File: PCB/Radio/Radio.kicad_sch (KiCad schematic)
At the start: 35 parts, among them J1 hc 12, J2 USB_C_Receptacle_USB2.0_16P, J3 seting, J4 config, J5 seting, J6 seting, J7 Conn_01x07_Pin, SW1 RotaryEncoder_Switch_MP, SW2 talk2push, SW3 SW_Push_45deg, SW4 SW_Push_45deg, SW5 SW_Push_45deg, SW6 SW_Push_45deg, SW7 RESET, SW8 RESET, U1 NRF24L01_Breakout, U2 ESP32-WROOM-32, U3 AMS1117-3.3, U4 CH340C

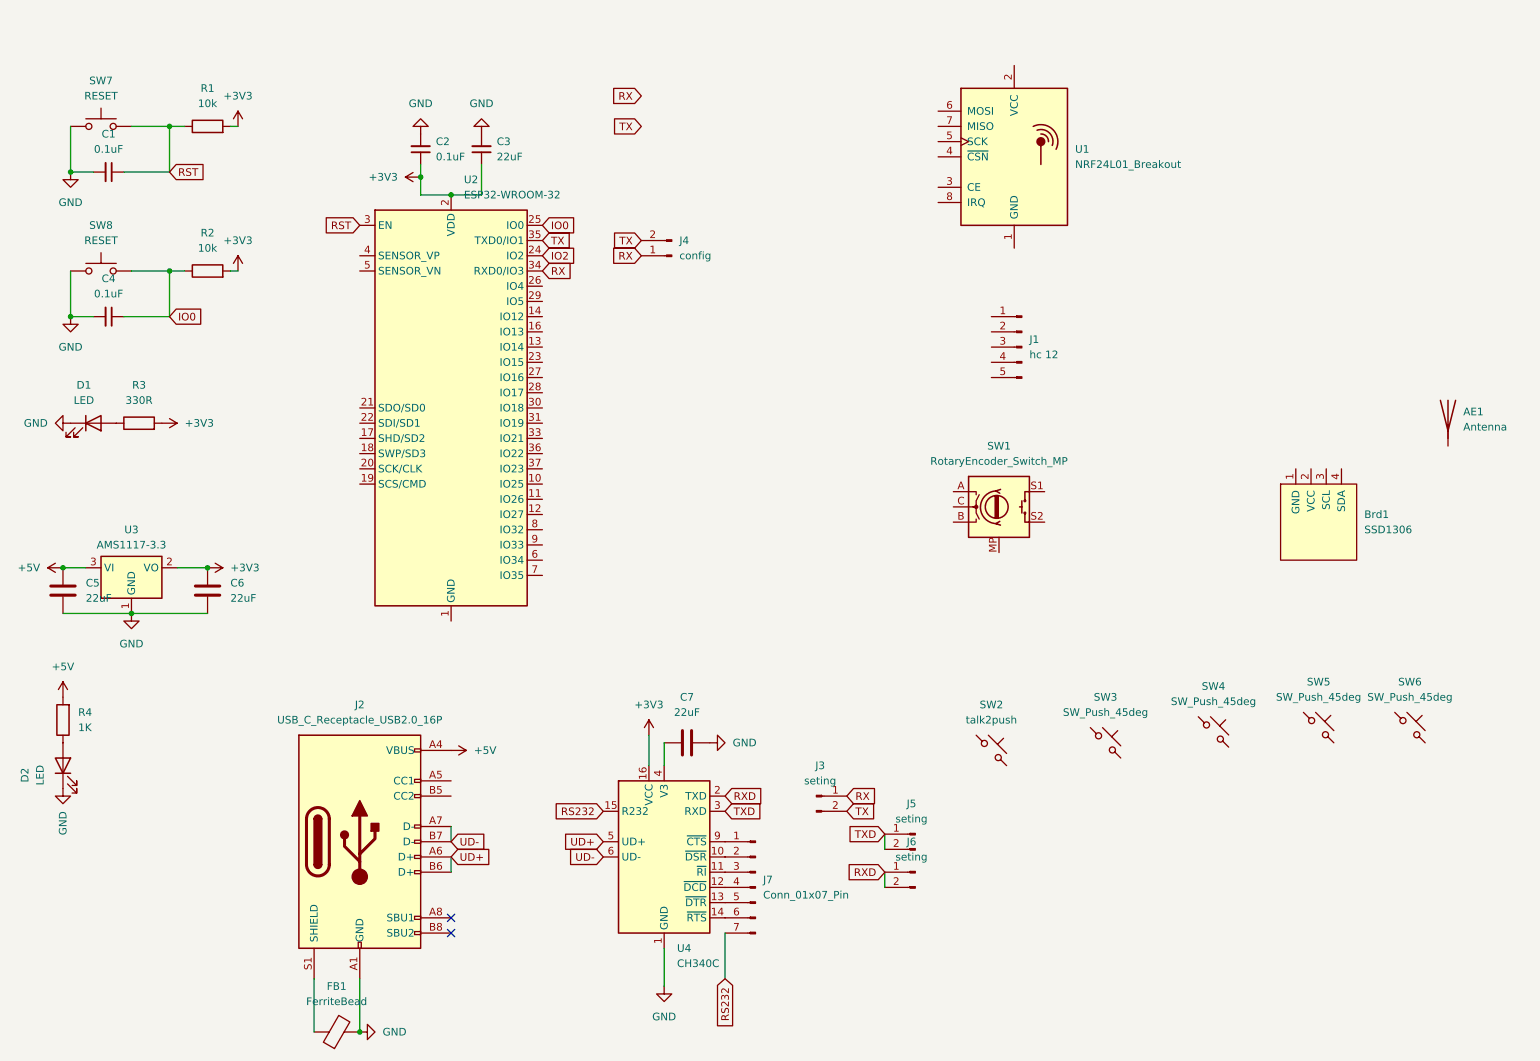
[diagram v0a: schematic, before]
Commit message: todays log
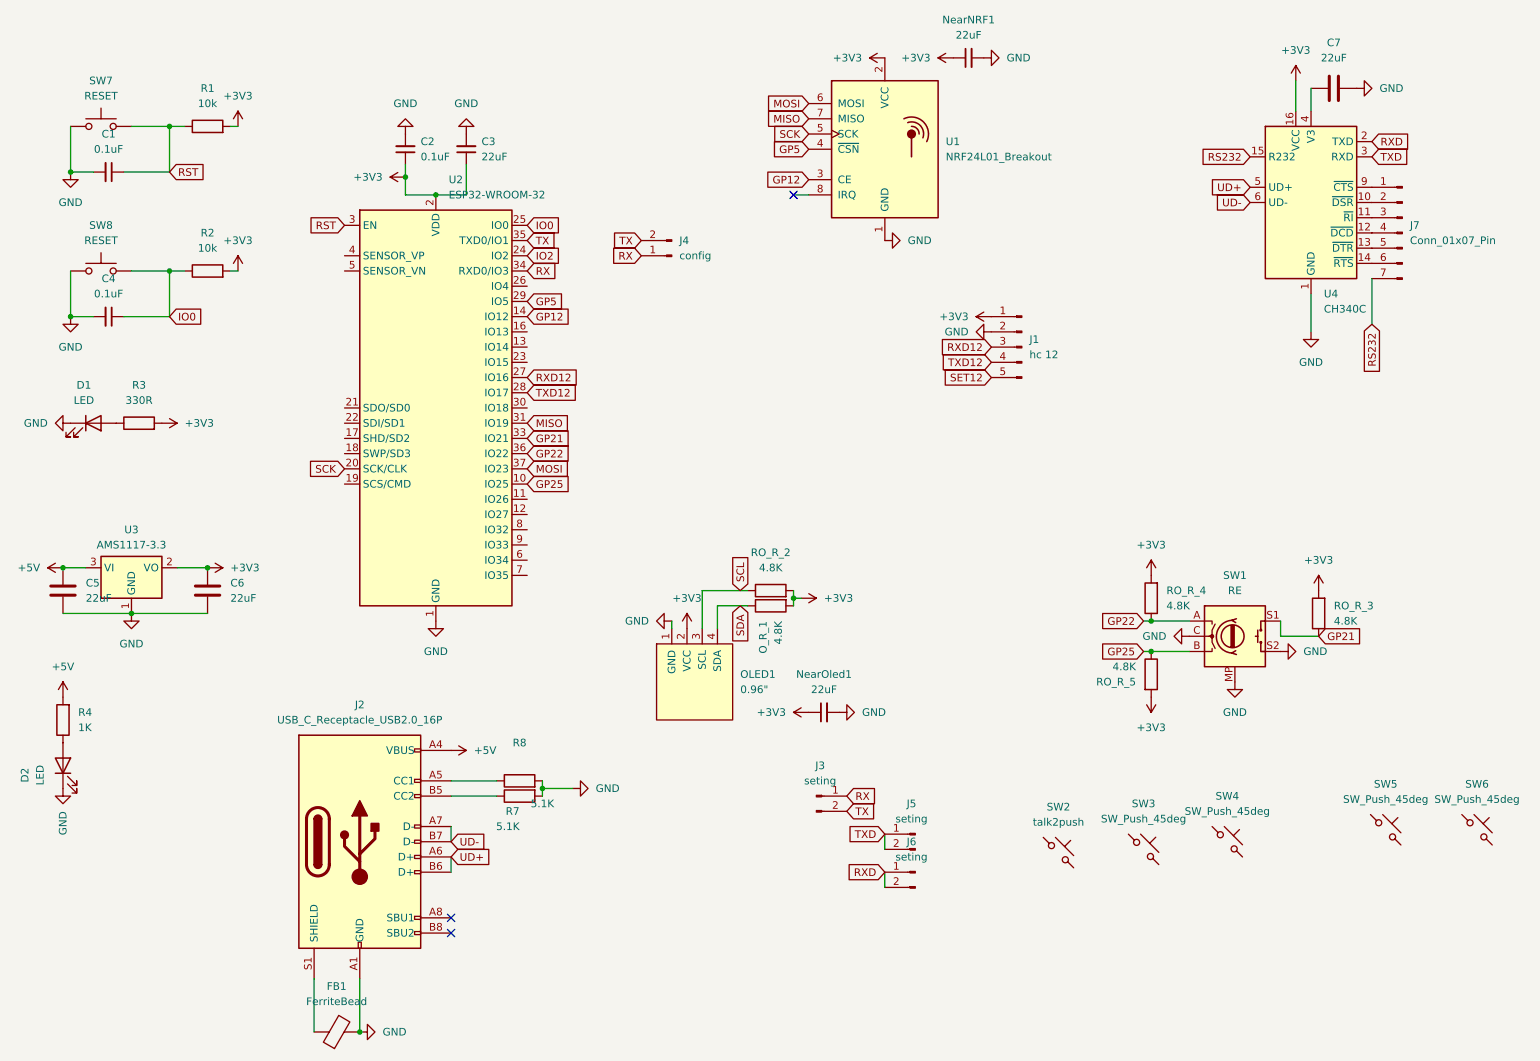
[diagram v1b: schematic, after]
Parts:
- removed AE1: Antenna, symbol Device:Antenna
- added NearNRF1, NearOled1: 22uF, Capacitor_SMD:C_1206_3216Metric_Pad1.33x1.80mm_HandSolder, symbol Device:C_Small
- added O_R_1, RO_R_2, RO_R_3, RO_R_4, RO_R_5: 4.8K, Resistor_THT:R_Axial_DIN0204_L3.6mm_D1.6mm_P7.62mm_Horizontal, symbol Device:R
- added R7, R8: 5.1K, Resistor_THT:R_Axial_DIN0204_L3.6mm_D1.6mm_P7.62mm_Horizontal, symbol Device:R
- C1, C2, C3, C4, C5, C6, C7: footprint (none) -> Capacitor_SMD:C_1206_3216Metric_Pad1.33x1.80mm_HandSolder
- D1, D2: footprint (none) -> LED_SMD:LED_1206_3216Metric_Pad1.42x1.75mm_HandSolder
- J3, J4, J5, J6: footprint (none) -> Connector_PinHeader_2.54mm:PinHeader_1x02_P2.54mm_Vertical
- J7: footprint (none) -> Connector_PinHeader_2.54mm:PinHeader_1x07_P2.54mm_Vertical
- OLED1: renamed from Brd1; value SSD1306 -> 0.96"; footprint (none) -> SSD1306:128x64OLED
- R1, R2, R3, R4: footprint (none) -> Resistor_THT:R_Axial_DIN0204_L3.6mm_D1.6mm_P7.62mm_Horizontal
- SW1: value RotaryEncoder_Switch_MP -> RE
- SW2, SW3, SW4, SW5, SW6, SW7, SW8: footprint (none) -> Button_Switch_THT:SW_PUSH_6mm
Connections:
- net +3V3: now also J1.1 (Pin_1), OLED1.2 (VCC), U1.2 (VCC), NearNRF1.1, NearOled1.1, O_R_1.2, RO_R_2.2, RO_R_3.2, RO_R_4.2, RO_R_5.2
- net GND: now also J1.2 (Pin_2), OLED1.1 (GND), SW1.C, SW1.MP, SW1.S2, U1.1 (GND), U2.1 (GND), U2.15 (GND), U2.38 (GND), U2.39 (GND), NearNRF1.2, NearOled1.2, R7.2, R8.2
- net GP25: now reaches U2.10 (IO25)
- net GP25: now also SW1.B, RO_R_5.1
- net GP12: now reaches U2.14 (IO12)
- net GP12: now also U1.3 (CE)
- net SCK: now reaches U2.20 (SCK/CLK)
- net SCK: now also U1.5 (SCK)
- net RXD12: now reaches U2.27 (IO16)
- net RXD12: now also J1.3 (Pin_3)
- net TXD12: now reaches U2.28 (IO17)
- net TXD12: now also J1.4 (Pin_4)
- net GP5: now reaches U2.29 (IO5)
- net GP5: now also U1.4 (~{CSN})
- net MISO: now reaches U2.31 (IO19)
- net MISO: now also U1.7 (MISO)
- net GP21: now reaches U2.33 (IO21)
- net GP21: now also SW1.S1, RO_R_3.1
- net GP22: now reaches U2.36 (IO22)
- net GP22: now also SW1.A, RO_R_4.1
- net MOSI: now reaches U2.37 (IO23)
- net MOSI: now also U1.6 (MOSI)
- net SCL: now reaches OLED1.3 (SCL)
- net SCL: now also RO_R_2.1
- net SDA: now reaches OLED1.4 (SDA)
- net SDA: now also O_R_1.1
- net at J2.A5 (CC1): now also R8.1
- net at J2.B5 (CC2): now also R7.1
- net SET12: now reaches J1.5 (Pin_5)
- no-connect marks 2 -> 3
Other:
- moved on the sheet: C2, C3, C7, J7, OLED1, SW1, SW2, SW3, SW4, SW5, SW6, U1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
